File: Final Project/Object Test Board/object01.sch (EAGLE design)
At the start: 18 parts, among them IC1 7805T, IC2 ATMEGA328P

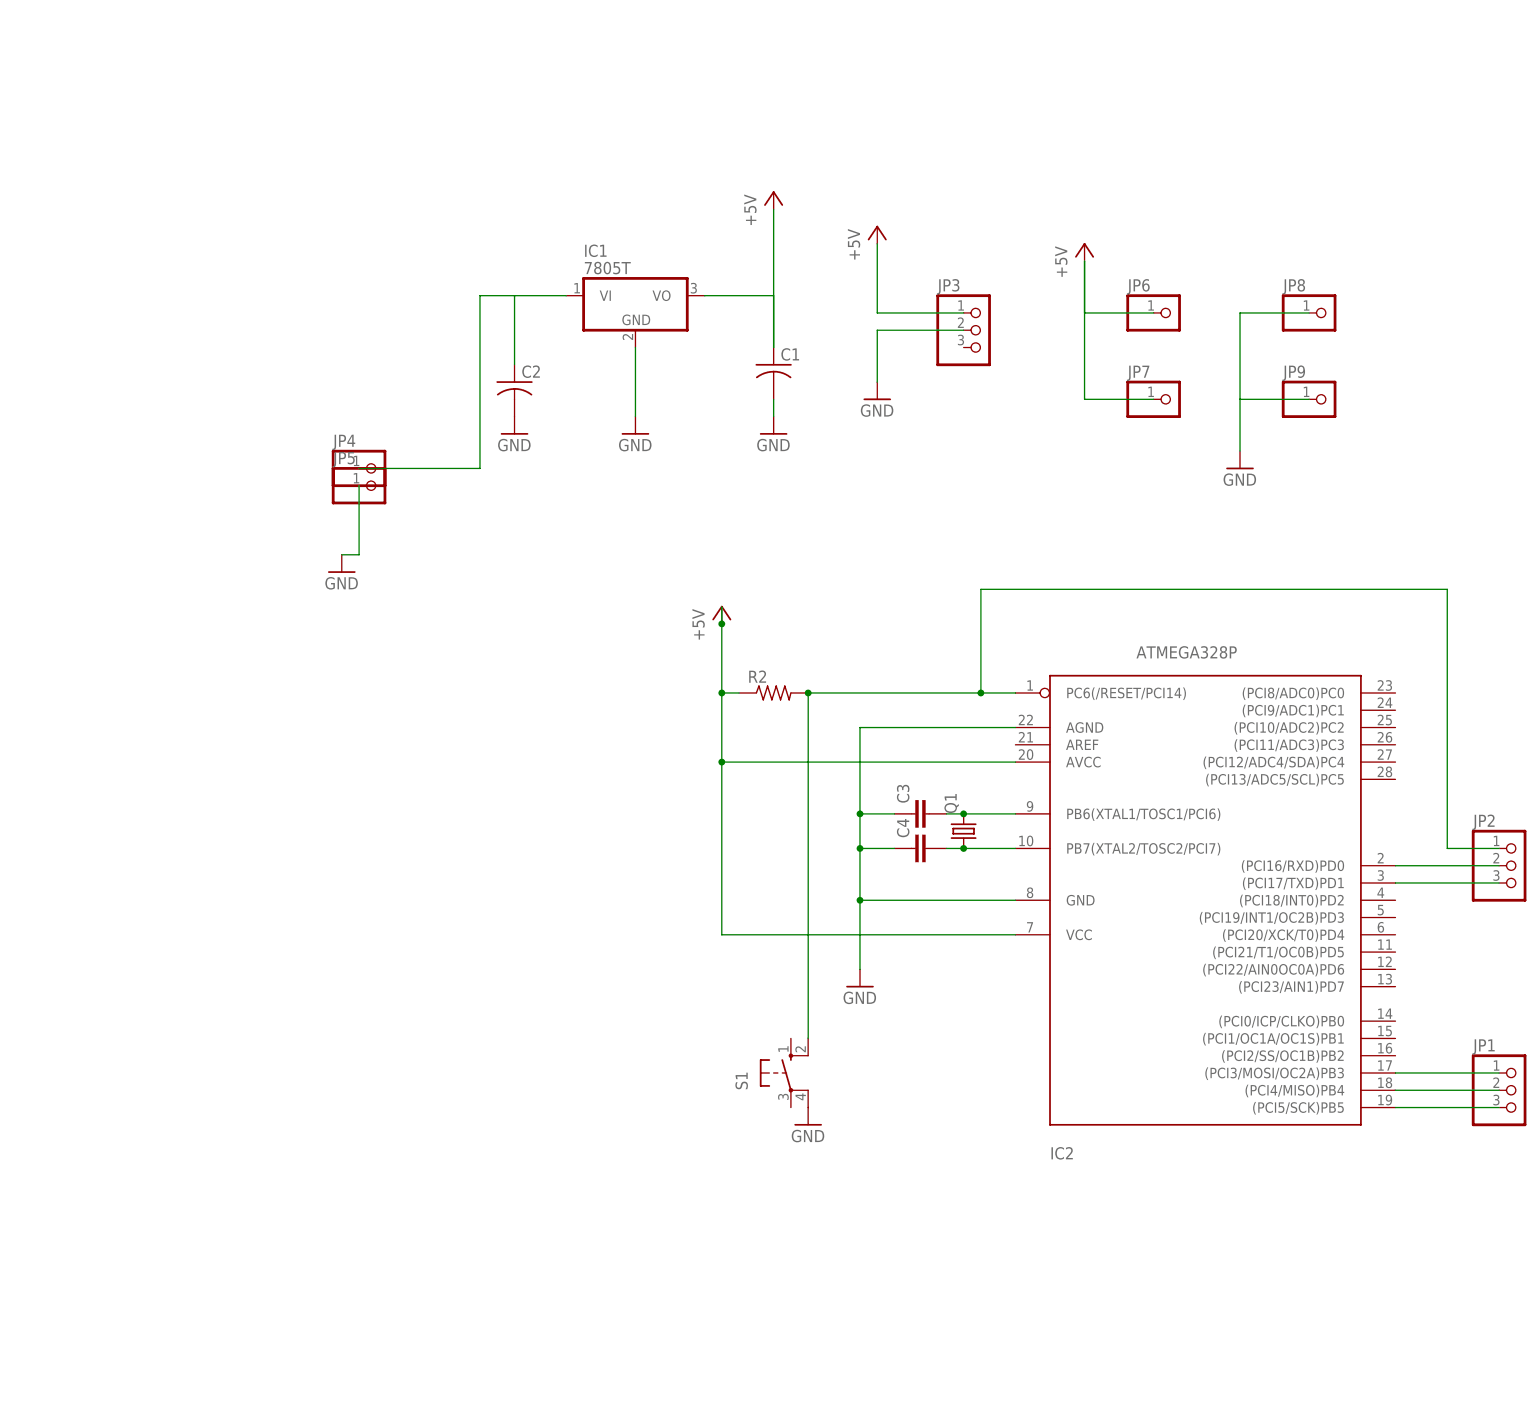
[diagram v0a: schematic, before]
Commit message: small edits to board
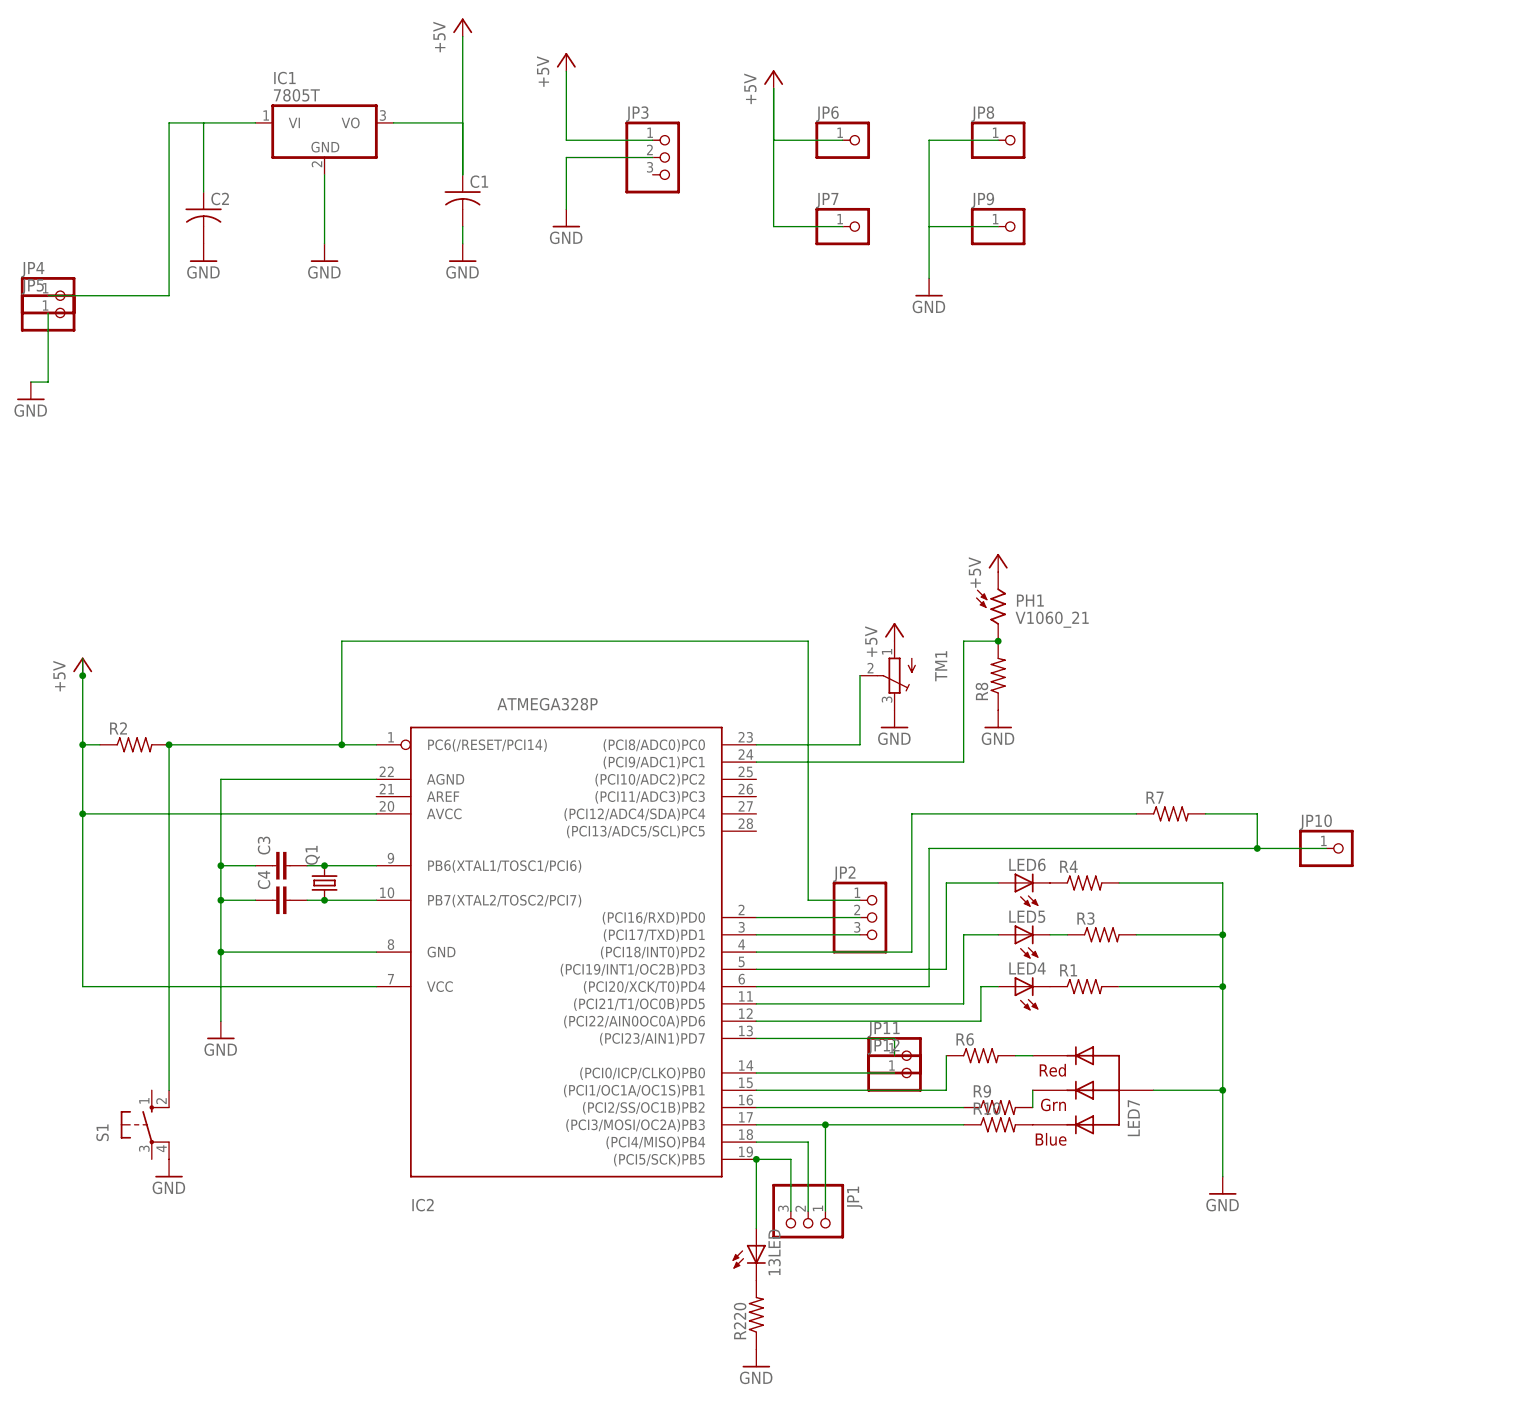
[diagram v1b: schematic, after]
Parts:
- added 13LED, LED4, LED5, LED6: (no value), led:LED5MM
- added JP10, JP11, JP12: (no value), adafruit:PINHD-1X1
- added LED7: RGBLED_CA-5MM, adafruit:RGBLED_CA-5MM
- added PH1: V1060_21, photo-elements:V1060_21
- added R1, R10, R220, R3, R4, R6, R7, R8, R9: (no value), resistor:R-US_0207/10
- added TM1: (no value), adafruit:TRIMPOT3386
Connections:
- new net N$10: LED7.RED, R6.2
- new net N$11: LED7.GREEN, R9.2
- new net N$12: LED5.C, R3.1
- new net N$13: LED4.C, R1.1
- new net N$14: LED6.C, R4.1
- new net N$16: IC2.(PCI0/ICP/CLKO)PB0, JP12.1
- new net N$17: IC2.(PCI19/INT1/OC2B)PD3, LED6.A
- new net N$18: IC2.(PCI21/T1/OC0B)PD5, LED5.A
- new net N$19: IC2.(PCI22/AIN0OC0A)PD6, LED4.A
- new net N$20: IC2.(PCI8/ADC0)PC0, TM1.S
- new net N$21: IC2.(PCI9/ADC1)PC1, PH1.2, R8.2
- new net N$22: IC2.(PCI23/AIN1)PD7, JP11.1
- new net N$23: IC2.(PCI18/INT0)PD2, R7.1
- new net N$24: IC2.(PCI20/XCK/T0)PD4, JP10.1, R7.2
- new net N$25: LED7.BLUE, R10.2
- new net N$26: 13LED.C, R220.2
- new net N$27: IC2.(PCI1/OC1A/OC1S)PB1, R6.1
- new net N$28: IC2.(PCI2/SS/OC1B)PB2, R9.1
- net +5V: now also PH1.1, TM1.A
- net GND: now also LED7.VCC, R1.2, R220.1, R3.2, R4.2, R8.1, TM1.E
- net N$4: now also R10.1
- net N$6: now also 13LED.A
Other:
- moved on the sheet: C1, C2, C3, C4, IC1, IC2, JP1, JP2, JP3, JP4, JP5, JP6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
